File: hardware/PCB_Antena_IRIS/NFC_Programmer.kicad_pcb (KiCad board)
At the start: 2 copper layers, 40 x 56.1 mm, 40 parts, among them J1 Conn_01x08, J2 Conn_01x02_Pin, U1 MFRC63002HN,151, Y1 Crystal_GND23

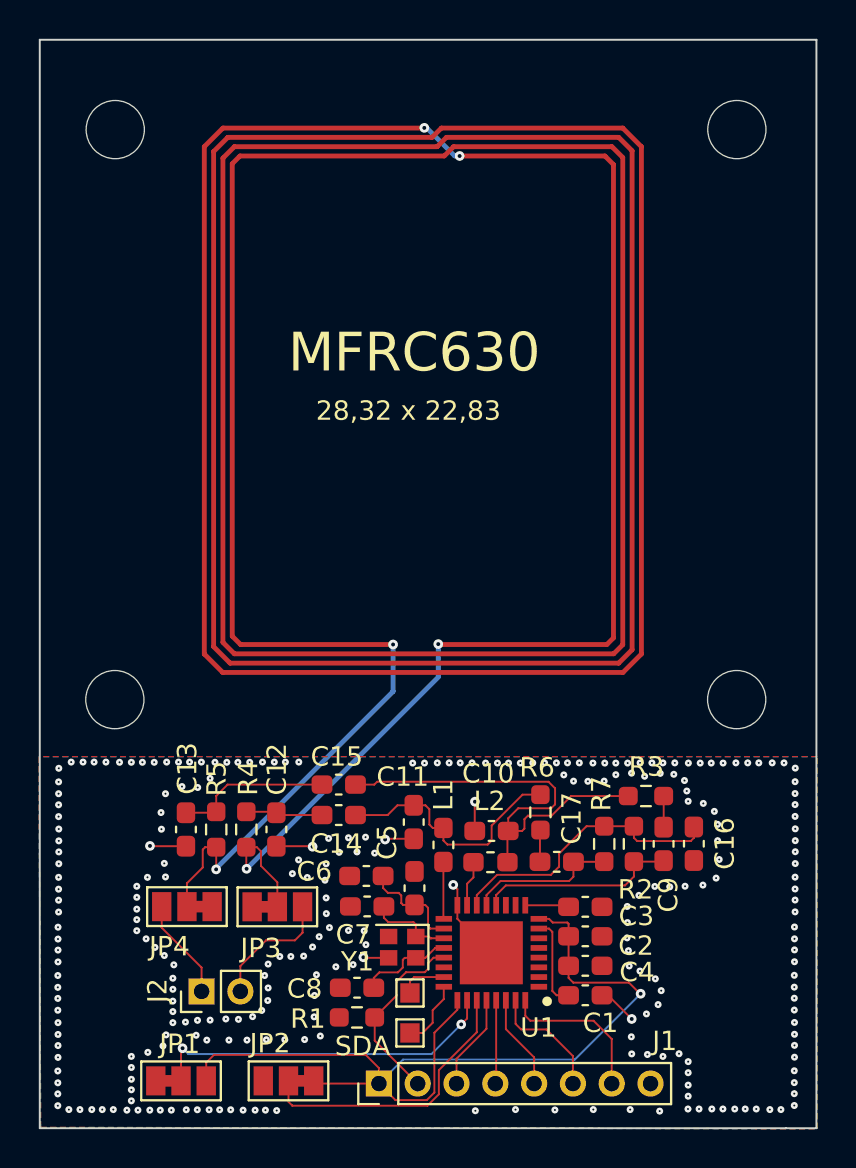
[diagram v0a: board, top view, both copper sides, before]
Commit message: Actualizacion
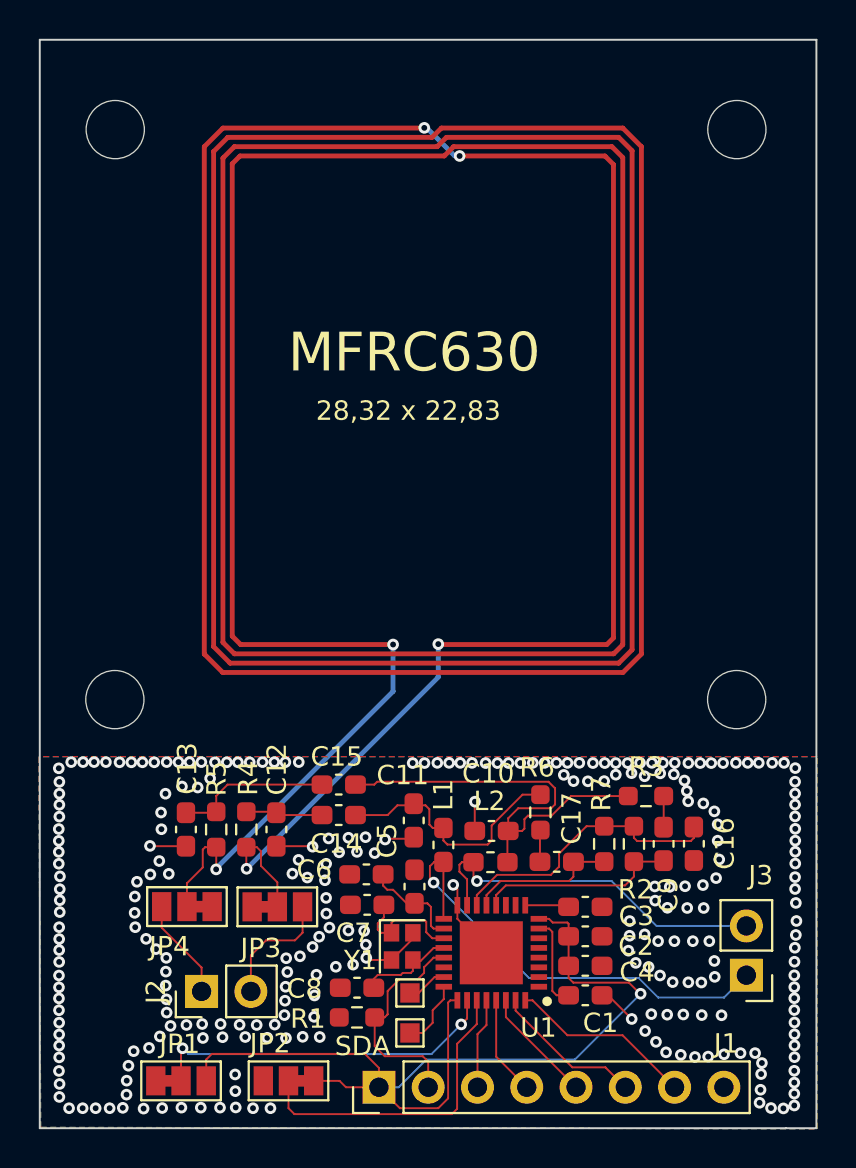
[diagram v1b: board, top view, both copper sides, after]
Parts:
- added J3: Conn_01x02_Pin, Connector_PinHeader_2.54mm:PinHeader_1x02_P2.54mm_Vertical, F.Cu at (156.6, 102.2)
- J1: footprint Connector_PinHeader_2.00mm:PinHeader_1x08_P2.00mm_Vertical -> Connector_PinHeader_2.54mm:PinHeader_1x08_P2.54mm_Vertical
- J2: footprint Connector_PinHeader_2.00mm:PinHeader_1x02_P2.00mm_Vertical -> Connector_PinHeader_2.54mm:PinHeader_1x02_P2.54mm_Vertical
- moved J1 0.19 mm to (137.7, 108.0)
- moved C7 0.08 mm to (137.1, 98.6)
- moved C11 0.08 mm to (139.5, 94.2)
- moved C5 0.08 mm to (139.5, 97.7)
- moved C6 0.08 mm to (137.0, 97.0)
- turned Y1 to -90 degrees
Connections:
- Y1 pad 3: GND -> Net-(U1-XTAL2)
- Y1 pad 4: Net-(U1-XTAL2) -> GND
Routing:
- net /TX1: track 2.94 -> 23.7 mm, vias 0 -> 1
- net /TX2: track 2.36 -> 18.9 mm, vias 0 -> 1
- net GND: track 14.4 -> 16.3 mm, vias 270 -> 262
- net /PDOWN: track 9.76 -> 11.6 mm
- net Net-(U1-XTAL1): track 4.49 -> 6.13 mm
- net +3V3: track 47.1 -> 48.6 mm
- net /IFSEL1: track 14.8 -> 16.4 mm
- net /NSS: track 6.28 -> 7.82 mm
- net /IRQ: track 8.05 -> 9.55 mm
- net /MISO: track 4.89 -> 5.98 mm
- net /SCK: track 4.31 -> 5.13 mm
